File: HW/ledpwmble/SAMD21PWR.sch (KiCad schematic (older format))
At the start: 7 parts

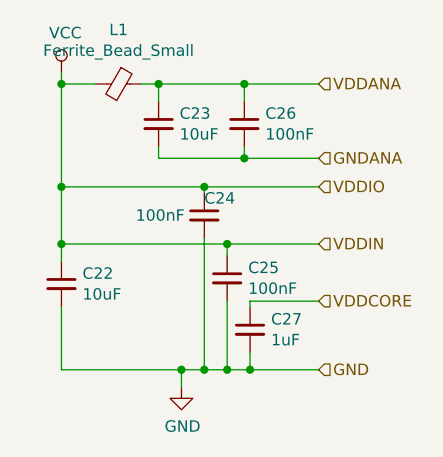
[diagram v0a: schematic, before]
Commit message: HW: Rev 1 - 1922
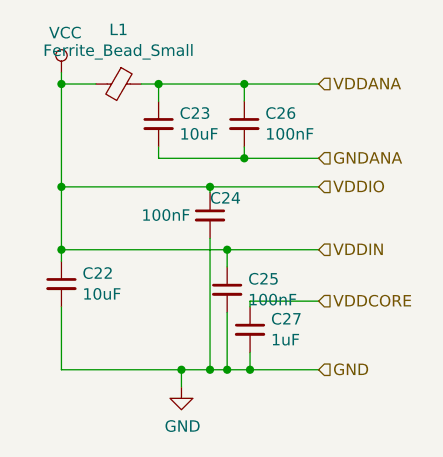
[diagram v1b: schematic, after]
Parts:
- C22, C23, C24, C25, C26, C27: footprint Capacitors_SMD:C_0805_HandSoldering -> Capacitor_SMD:C_0603_1608Metric
- L1: footprint Capacitors_SMD:C_0603_HandSoldering -> Inductor_SMD:L_0603_1608Metric
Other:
- moved on the sheet: C24, C25
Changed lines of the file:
@@
 $Descr A4 11693 8268
 encoding utf-8
-Sheet 4 3
+Sheet 3 3
 Title ""
 Date ""
@@
 F 0 "L1" V 3388 2900 50  0000 C CNN
 F 1 "Ferrite_Bead_Small" V 3479 2900 50  0000 C CNN
-F 2 "Capacitors_SMD:C_0603_HandSoldering" V 3555 2900 50  0001 C CNN
+F 2 "Inductor_SMD:L_0603_1608Metric" V 3555 2900 50  0001 C CNN
 F 3 "" H 3625 2900 50  0001 C CNN
 	1    3625 2900
@@
 F 0 "C23" H 3892 3121 50  0000 L CNN
 F 1 "10uF" H 3892 3030 50  0000 L CNN
-F 2 "Capacitors_SMD:C_0805_HandSoldering" H 3800 3075 50  0001 C CNN
+F 2 "Capacitor_SMD:C_0603_1608Metric" H 3800 3075 50  0001 C CNN
 F 3 "" H 3800 3075 50  0001 C CNN
 	1    3800 3075
@@
 F 0 "C26" H 4267 3121 50  0000 L CNN
 F 1 "100nF" H 4267 3030 50  0000 L CNN
-F 2 "Capacitors_SMD:C_0805_HandSoldering" H 4175 3075 50  0001 C CNN
+F 2 "Capacitor_SMD:C_0603_1608Metric" H 4175 3075 50  0001 C CNN
 F 3 "" H 4175 3075 50  0001 C CNN
 	1    4175 3075
@@
 Wire Wire Line
 	4175 3225 4500 3225
-$Comp
-L Device:C_Small C24
-U 1 1 5B0514CB
-P 4000 3475
-F 0 "C24" H 4000 3550 50  0000 L CNN
-F 1 "100nF" H 3700 3475 50  0000 L CNN
-F 2 "Capacitors_SMD:C_0805_HandSoldering" H 4000 3475 50  0001 C CNN
-F 3 "" H 4000 3475 50  0001 C CNN
-	1    4000 3475
-	1    0    0    -1
-$EndComp
-Wire Wire Line
-	4000 3375 4000 3350
-Wire Wire Line
-	4000 3350 4500 3350
 Wire Wire Line
 	4500 4150 4200 4150
@@
 F 0 "C22" H 3467 3821 50  0000 L CNN
 F 1 "10uF" H 3467 3730 50  0000 L CNN
-F 2 "Capacitors_SMD:C_0805_HandSoldering" H 3375 3775 50  0001 C CNN
+F 2 "Capacitor_SMD:C_0603_1608Metric" H 3375 3775 50  0001 C CNN
 F 3 "" H 3375 3775 50  0001 C CNN
 	1    3375 3775
@@
 $EndComp
 Wire Wire Line
-	3375 3675 3375 3600
+	3375 3675 3375 3625
 Connection ~ 3375 2900
-Wire Wire Line
-	4000 3350 3375 3350
-Connection ~ 4000 3350
 Connection ~ 3375 3350
 Wire Wire Line
 	3375 3350 3375 2900
-Wire Wire Line
-	4000 3575 4000 4150
-Connection ~ 4000 4150
-Wire Wire Line
-	4000 4150 3900 4150
 $Comp
 L power:GND #PWR047
@@
 L Device:C_Small C25
 U 1 1 5B0514F0
-P 4100 3750
-F 0 "C25" H 4192 3796 50  0000 L CNN
-F 1 "100nF" H 4192 3705 50  0000 L CNN
-F 2 "Capacitors_SMD:C_0805_HandSoldering" H 4100 3750 50  0001 C CNN
-F 3 "" H 4100 3750 50  0001 C CNN
-	1    4100 3750
-	1    0    0    -1
-$EndComp
-Wire Wire Line
-	4100 3650 4100 3600
-Wire Wire Line
-	4100 3600 4500 3600
-Wire Wire Line
-	4100 3600 3375 3600
-Connection ~ 4100 3600
-Connection ~ 3375 3600
-Wire Wire Line
-	3375 3600 3375 3350
-Wire Wire Line
-	4100 3850 4100 4150
+P 4100 3800
+F 0 "C25" H 4192 3846 50  0000 L CNN
+F 1 "100nF" H 4192 3755 50  0000 L CNN
+F 2 "Capacitor_SMD:C_0603_1608Metric" H 4100 3800 50  0001 C CNN
+F 3 "" H 4100 3800 50  0001 C CNN
+	1    4100 3800
+	1    0    0    -1
+$EndComp
+Wire Wire Line
+	4100 3700 4100 3625
+Wire Wire Line
+	4100 3625 4500 3625
+Connection ~ 4100 3625
+Connection ~ 3375 3625
+Wire Wire Line
+	3375 3625 3375 3350
+Wire Wire Line
+	4100 3900 4100 4150
 Connection ~ 4100 4150
-Wire Wire Line
-	4100 4150 4000 4150
 $Comp
 L Device:C_Small C27
@@
 F 0 "C27" H 4292 4021 50  0000 L CNN
 F 1 "1uF" H 4292 3930 50  0000 L CNN
-F 2 "Capacitors_SMD:C_0805_HandSoldering" H 4200 3975 50  0001 C CNN
+F 2 "Capacitor_SMD:C_0603_1608Metric" H 4200 3975 50  0001 C CNN
 F 3 "" H 4200 3975 50  0001 C CNN
 	1    4200 3975
@@
 Text HLabel 4500 4150 2    50   Input ~ 0
 GND
-Text HLabel 4500 3600 2    50   Input ~ 0
+Text HLabel 4500 3625 2    50   Input ~ 0
 VDDIN
+Wire Wire Line
+	3900 4150 4025 4150
+$Comp
+L Device:C_Small C24
+U 1 1 5B0514CB
+P 4025 3475
+F 0 "C24" H 4025 3550 50  0000 L CNN
+F 1 "100nF" H 3725 3475 50  0000 L CNN
+F 2 "Capacitor_SMD:C_0603_1608Metric" H 4025 3475 50  0001 C CNN
+F 3 "" H 4025 3475 50  0001 C CNN
+	1    4025 3475
+	1    0    0    -1
+$EndComp
+Wire Wire Line
+	3375 3350 4025 3350
+Wire Wire Line
+	4025 3375 4025 3350
+Connection ~ 4025 3350
+Wire Wire Line
+	4025 3350 4500 3350
+Wire Wire Line
+	3375 3625 4100 3625
+Wire Wire Line
+	4025 3575 4025 4150
+Connection ~ 4025 4150
+Wire Wire Line
+	4025 4150 4100 4150
 $EndSCHEMATC
